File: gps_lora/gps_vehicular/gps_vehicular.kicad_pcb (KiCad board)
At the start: 2 copper layers, 71.1 x 41.3 mm, 53 parts, among them J1 IN 12V, J2 USB_B, J3 ADJ, J4 BAT, J5 IGN, J6 RELAY, J7 PANI, J8 SWD, Q1 Q_PMOS_GSD, Q2 SMMBT3904LT1G, Q3 SMMBT3904LT1G, SW1 RST, U1 LM2596, U2 AP2114-3.3, U3 MCP73831-3-OT, U4 LTV-352T, U5 LTV-352T, U6 ATSAMD21E, U7 LTV-352T, U8 RFM95W-868S2

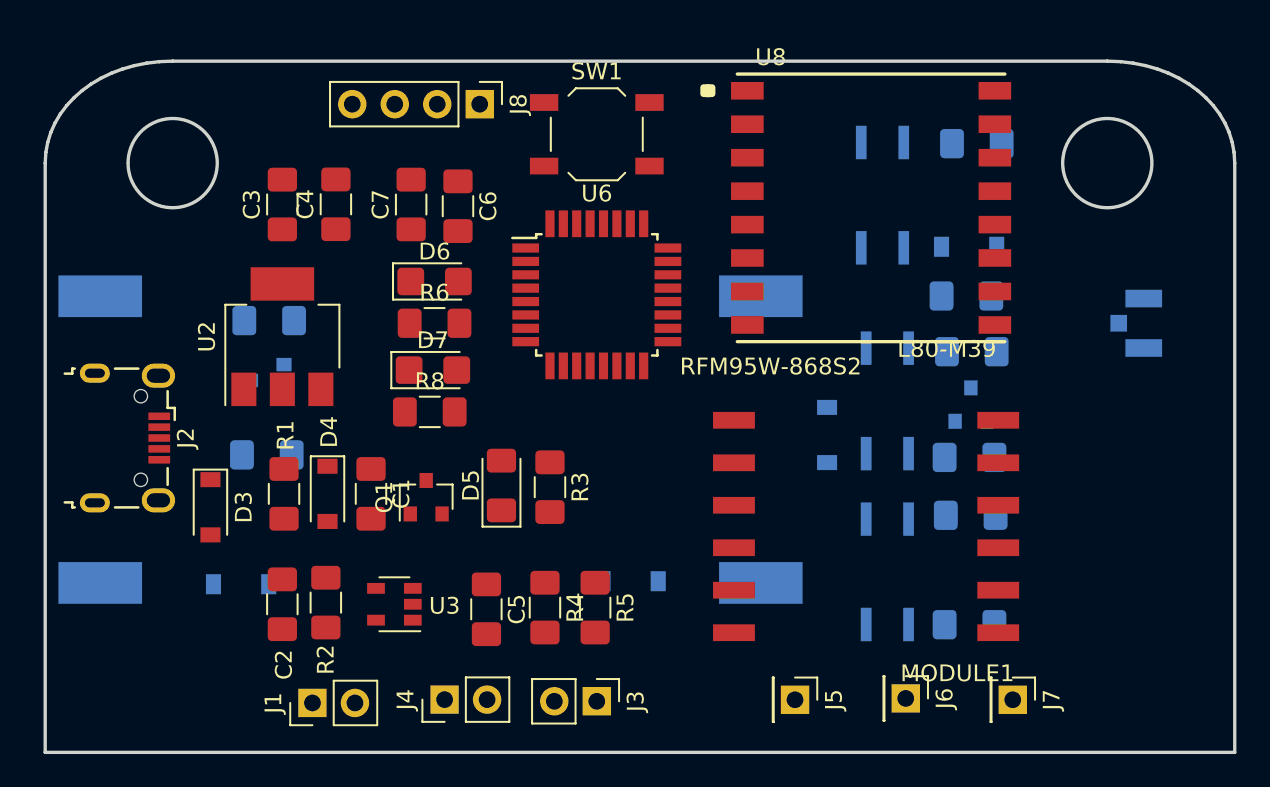
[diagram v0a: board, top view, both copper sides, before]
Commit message: add pcb gps vehicular and minimo
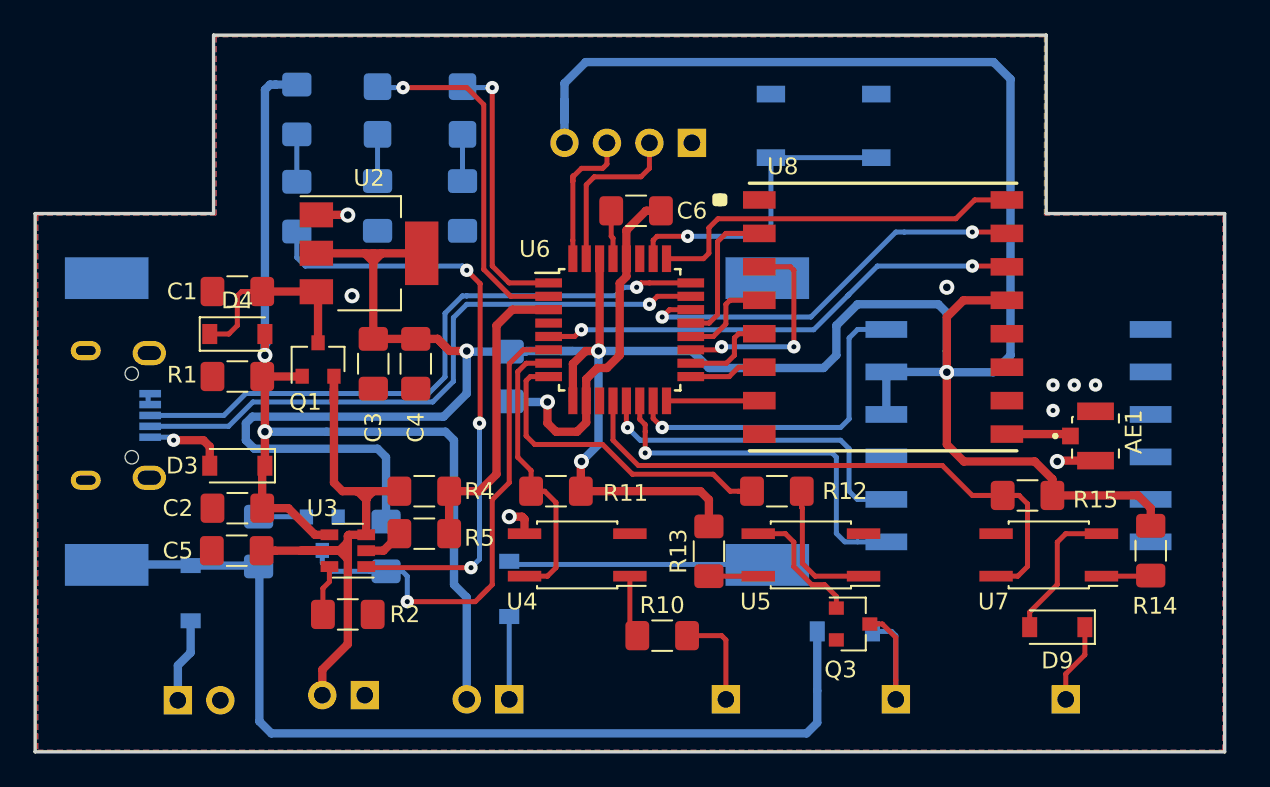
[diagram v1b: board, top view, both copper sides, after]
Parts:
- AE1, D9, Q3, R10, R11, R12, R13, R14, R15, U4, U5, U7: moved to F.Cu
- C7, D5, D6, D7, J1, J2, J3, J4, J5, J6, J7, J8, MODULE1, R3, R6, R8, SW1: moved to B.Cu
- moved D5 25.6 mm to (118.4, 55.9)
- moved R11 24.8 mm to (133.9, 78.7)
- moved U7 23.7 mm to (163.3, 82.5), turned to 180 degrees
- moved D9 23.3 mm to (163.8, 86.9)
- moved R3 22.6 mm to (118.4, 61.7)
- moved R15 21.3 mm to (162.1, 79.0)
- moved R13 19.7 mm to (143.0, 82.3), turned to 90 degrees
- moved R14 18.8 mm to (169.4, 82.3), turned to 90 degrees
- moved U4 18.6 mm to (135.1, 82.5), turned to 180 degrees
- moved R10 18.4 mm to (140.2, 87.4)
- moved D7 15.9 mm to (123.2, 56.0), turned to 90 degrees
- moved C5 15.3 mm to (114.8, 82.3), turned to 180 degrees
- moved R9 15.2 mm to (123.7, 82.0), turned to 90 degrees
- moved Q3 14.9 mm to (151.6, 86.7), turned to 0 degrees
- moved C1 14.5 mm to (114.8, 66.8), turned to 180 degrees
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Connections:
- U6 pad 1: Net-(U6-Pad1) -> /microcontroller/LED_1
- U6 pad 12: Net-(U6-Pad12) -> /microcontroller/SIG_PANI
- U6 pad 15: Net-(U6-Pad15) -> /microcontroller/1PPS
- U6 pad 2: Net-(U6-Pad2) -> /microcontroller/LED_2
- U6 pad 6: Net-(U6-Pad6) -> /microcontroller/SIG_CONECTADO
- U6 pad 7: Net-(U6-Pad7) -> /microcontroller/SIG_IGNI
- U6 pad 8: Net-(U6-Pad8) -> /microcontroller/OUT_SIG
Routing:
- net +3V3: track 0.00 -> 200.1 mm, vias 0 -> 4
- net +5V: track 0.00 -> 63.7 mm, vias 0 -> 2
- net +12V: track 0.00 -> 58.5 mm
- net D+: track 0.00 -> 37.8 mm, vias 0 -> 1
- net D-: track 0.00 -> 37.8 mm, vias 0 -> 1
- net +BATT: track 0.00 -> 37.8 mm
- net Net-(R3-Pad2): track 0.00 -> 36.7 mm, vias 0 -> 3
- net /microcontroller/SIG_PANI: track 0.00 -> 35.6 mm
- net /microcontroller/SIG_CONECTADO: track 0.00 -> 30.8 mm, vias 0 -> 1
- net /microcontroller/DIO0: track 0.00 -> 29.3 mm, vias 0 -> 2
- net GND: track 0.00 -> 27.8 mm, vias 0 -> 9
- net /microcontroller/DIO1: track 0.00 -> 24.6 mm, vias 0 -> 2
- net /microcontroller/DIO2: track 0.00 -> 22.7 mm
- net /microcontroller/RX_GPS: track 0.00 -> 22.5 mm, vias 0 -> 1
- net /microcontroller/LED_2: track 0.00 -> 21.2 mm, vias 0 -> 1
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- added copper zone on B.Cu, net GND
- added copper zone on F.Cu, net GND
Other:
- board size 71.1 x 41.3 mm -> 71.1 x 42.8 mm
- net class Default: trace_width 0.25 -> 0.3; via_drill 0.4 -> 0.3
- net class Source added: clearance 0.2, trace_width 0.5, via_dia 0.9, via_drill 0.45
- board text added: "+"
- board text added: "-"
- board text added: "1"
